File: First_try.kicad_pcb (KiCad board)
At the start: 4 copper layers, 58.1 x 62.5 mm, 136 parts, among them J1 TYPE-611-T3-W, J10 Conn_01x11, J2 Conn_01x02, J3 Conn_01x02, J4 Conn_01x11, J5 Conn_01x02, J6 Conn_01x02, J7 Conn_01x02, J9 Conn_01x02, SW1 SW_Push, SW2 SW_Push, SW3 SW_Push, SW7 EG1218, U1 FT232HL-REEL, U10 20m, U11 20m, U2 TPS62026DRCR, U3 SN74AUP2G125DCUR, U4 INA226AIDGSR, U5 INA226AIDGSR, U6 93LC56BT-I/OT, U7 ICE40UP5K-SG48I, U8 W25Q32JVSSIQ

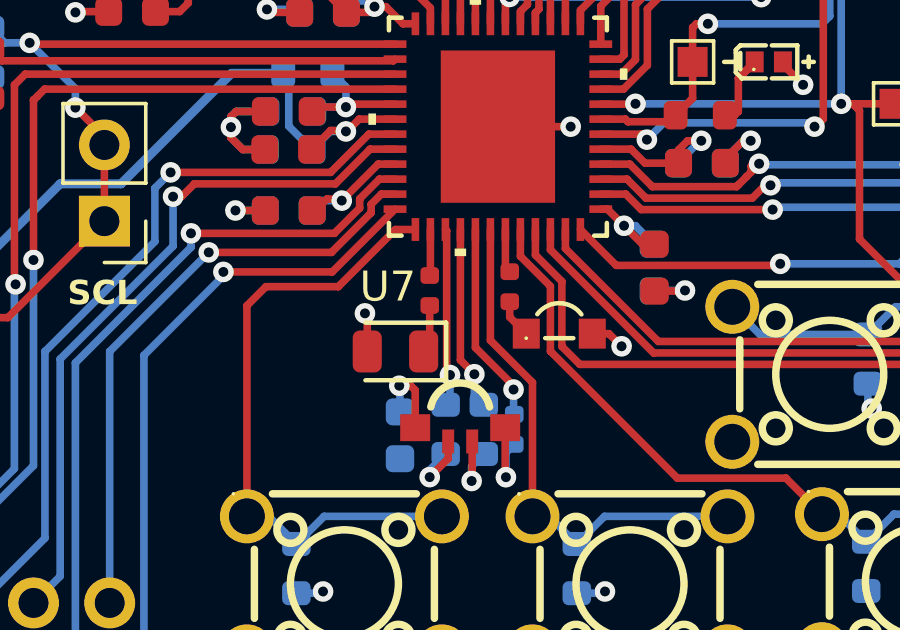
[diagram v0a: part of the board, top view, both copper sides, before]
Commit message: RISC-V added
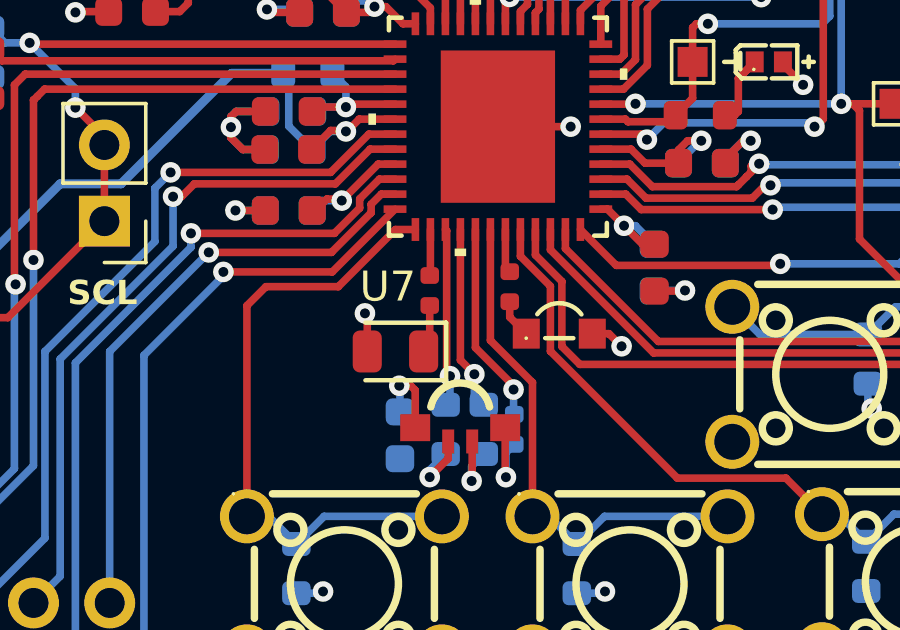
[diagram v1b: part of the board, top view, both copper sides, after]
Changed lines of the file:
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@@
 	)
 	(segment
-		(start 227.5986 65.9122)
-		(end 227.641 65.9546)
-		(width 0.254)
-		(layer "F.Cu")
-		(net 58)
-	)
-	(segment
-		(start 227.641 65.9546)
+		(start 227.751857 70.762361)
 		(end 227.641 70.651504)
 		(width 0.254)
@@
 	(segment
 		(start 227.641 70.651504)
+		(end 227.641 65.9546)
+		(width 0.254)
+		(layer "F.Cu")
+		(net 58)
+	)
+	(segment
+		(start 227.751857 70.8)
 		(end 227.751857 70.762361)
 		(width 0.254)
@@
 		(net 58)
 	)
+	(segment
+		(start 227.641 65.9546)
+		(end 227.5986 65.9122)
+		(width 0.254)
+		(layer "F.Cu")
+		(net 58)
+	)
 	(via
-		(at 227.751857 70.762361)
+		(at 227.751857 70.8)
 		(size 0.6858)
 		(drill 0.3302)
@@
 	)
 	(segment
-		(start 227.751857 70.762361)
+		(start 227.751857 70.8)
 		(end 227.751857 71.611143)
 		(width 0.254)
